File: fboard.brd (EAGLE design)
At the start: 60.9 x 51.7 mm, 29 parts, among them Q1 SL2305, U1 ATMEGA328PB-AU, U2 MPU-6050, U3 SN74HC138PW

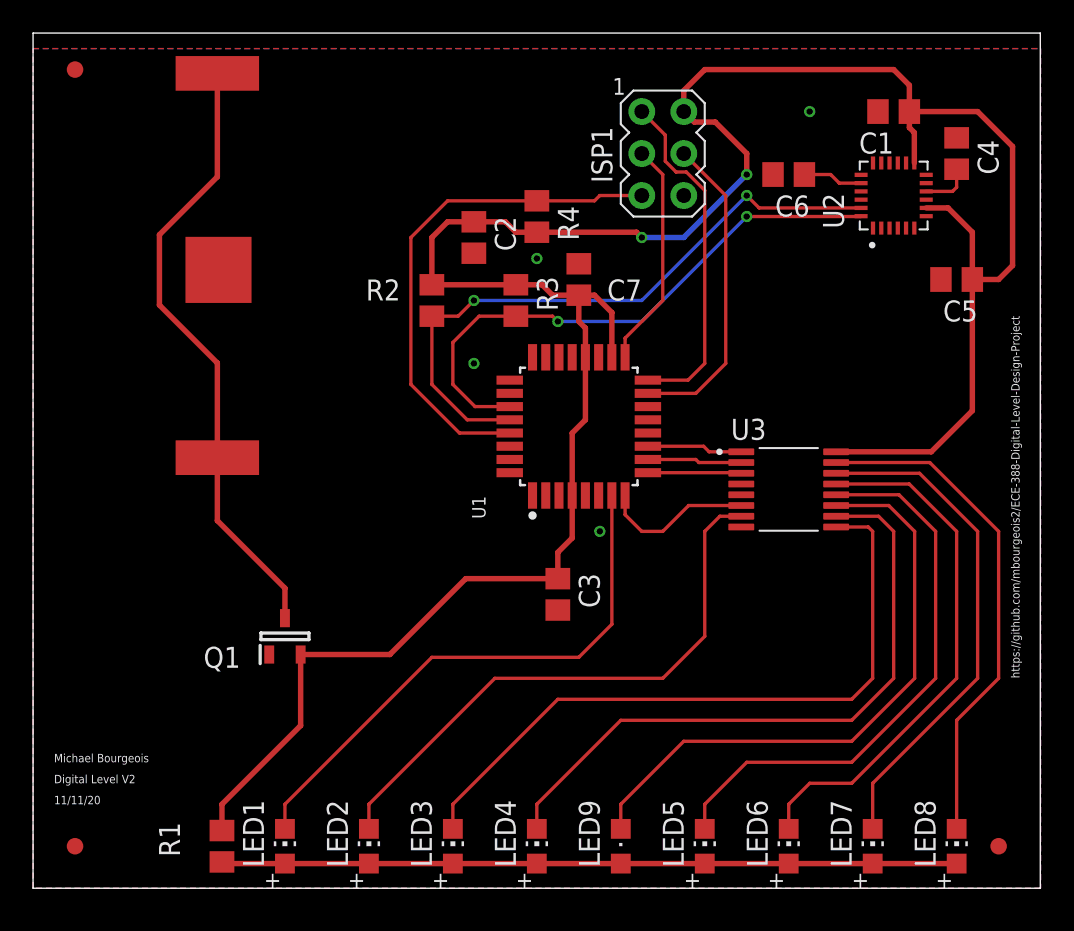
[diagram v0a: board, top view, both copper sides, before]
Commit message: added easter egg
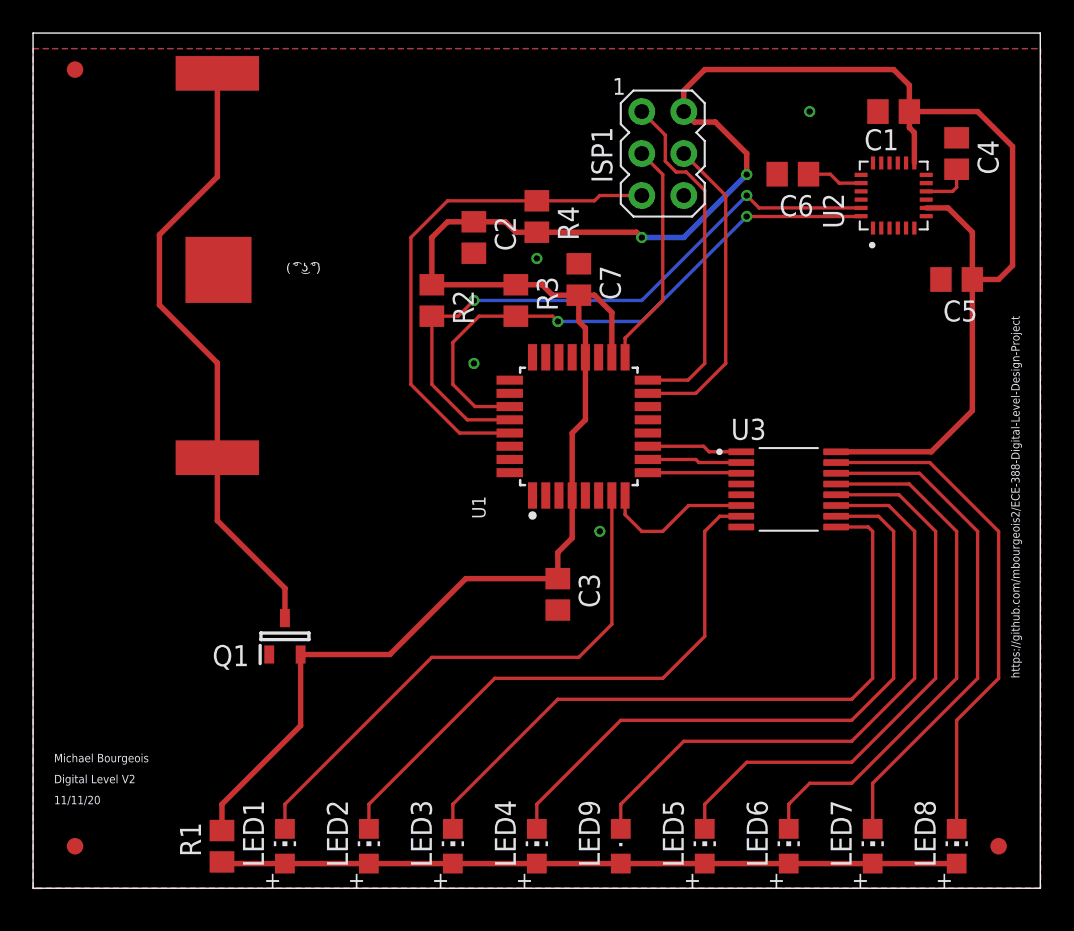
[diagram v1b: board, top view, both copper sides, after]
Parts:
- moved C6 0.25 mm to (46.0, 43.2)
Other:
- board text added: "C:/Users/Michael/Desktop/lenny.bmp"
